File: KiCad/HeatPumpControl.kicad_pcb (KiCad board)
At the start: 2 copper layers, 36.6 x 38.9 mm, 43 parts, among them J1 Conn_01x04_Male, J2 Conn_01x04_Male, J3 Conn_01x04_Male, J4 Conn_01x03_Male, Q1 2N2222A, Q2 Q_PMOS_GDS, U3 XIAO-ESP32-C6-SMD

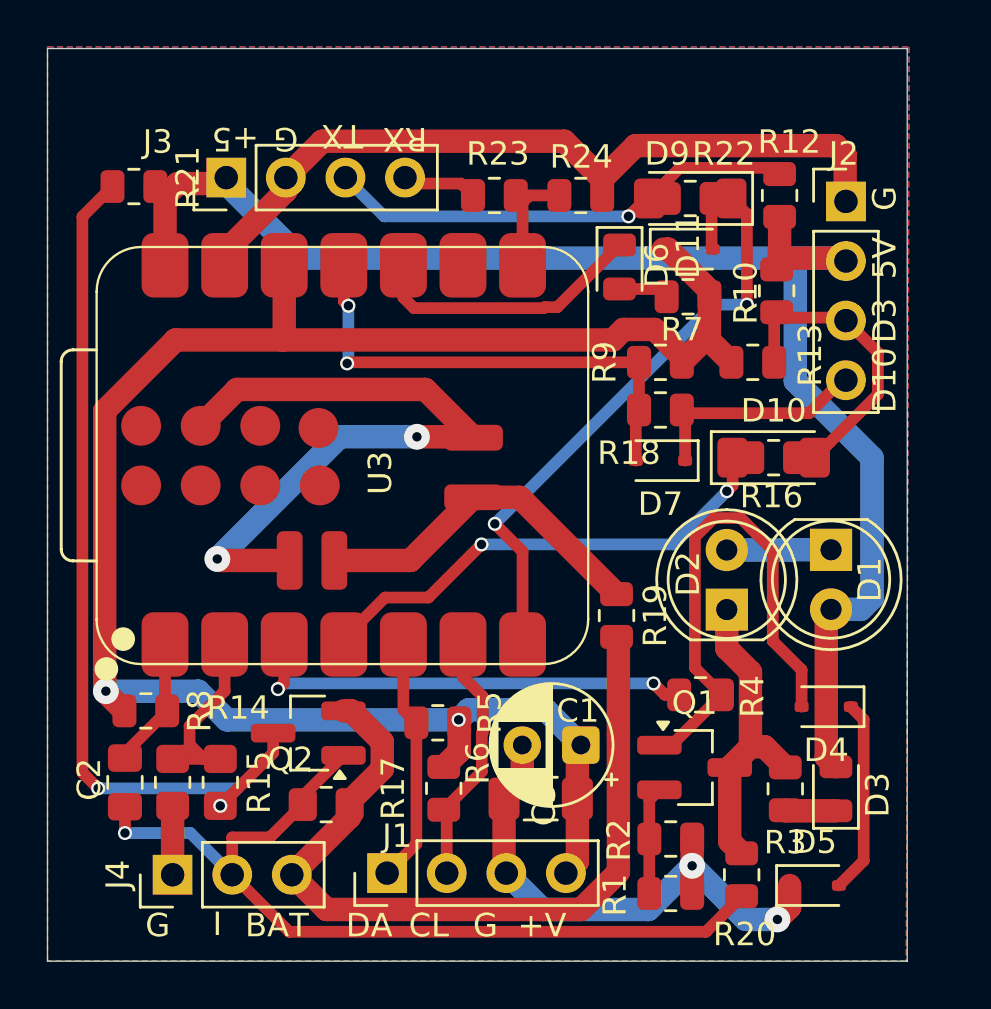
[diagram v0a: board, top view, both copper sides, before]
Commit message: Manufacturing for v4.0
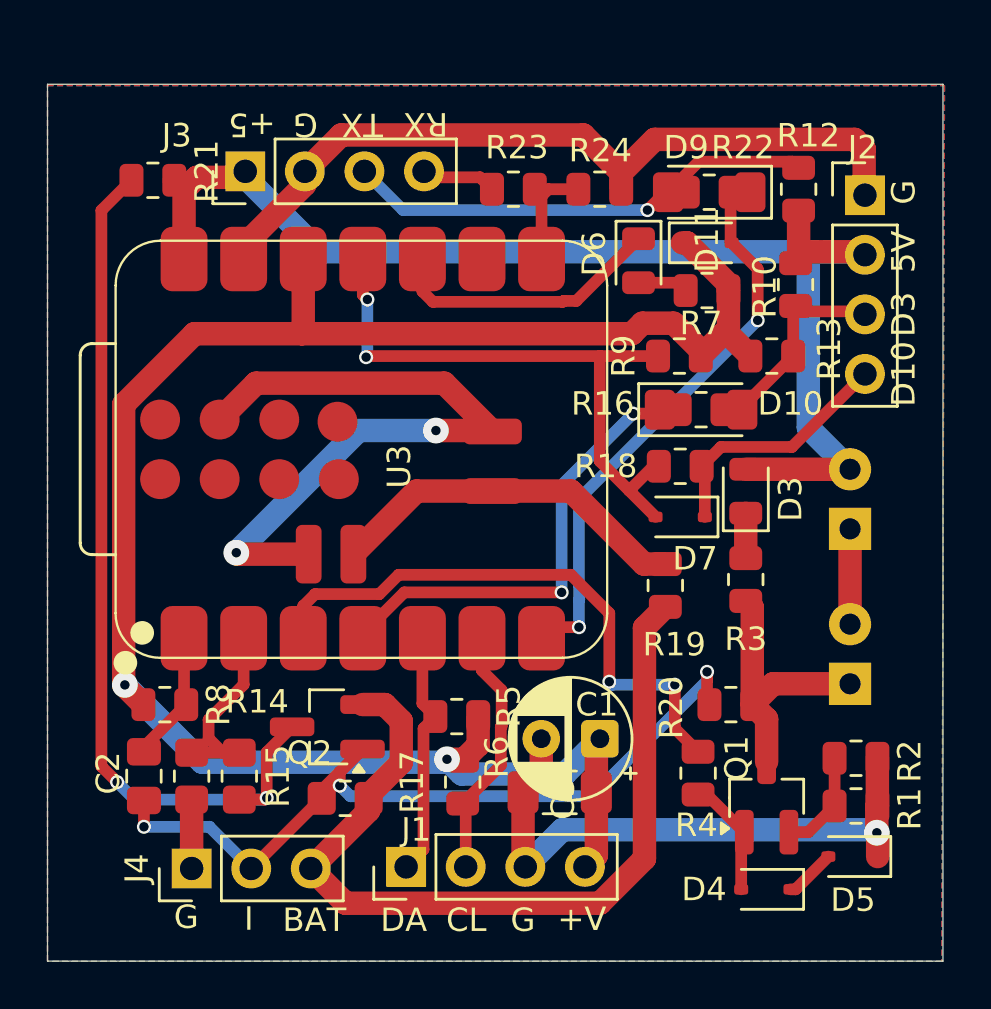
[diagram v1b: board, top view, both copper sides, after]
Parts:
- D1, D2: moved to B.Cu
- moved D3 13.3 mm to (165.7, 103.8)
- moved R3 9.08 mm to (165.7, 107.6), turned to 90 degrees
- moved R1 8.73 mm to (170.4, 117.2)
- moved R2 8.62 mm to (170.4, 115.2)
- moved D4 8.20 mm to (166.5, 120.8)
- moved R20 7.27 mm to (165.0, 112.9), turned to 0 degrees
- moved D2 6.13 mm to (170.1, 112.0)
- moved D10 3.71 mm to (163.8, 100.3)
- moved R16 3.71 mm to (163.8, 100.3)
- moved R4 3.34 mm to (163.6, 115.8), turned to -90 degrees
- moved Q1 3.32 mm to (166.5, 116.8), turned to 90 degrees
- moved D7 2.54 mm to (162.9, 104.9)
- moved R18 2.54 mm to (162.9, 102.7)
- moved R19 2.44 mm to (162.2, 107.8)
- moved D5 2.06 mm to (170.2, 119.4), turned to 180 degrees
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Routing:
- net Net-(D4-A): track 22.2 -> 5.13 mm
- net +5V: track 63.9 -> 53.6 mm
- net Net-(D4-K): track 8.28 -> 2.20 mm
- net /D10: track 21.0 -> 26.3 mm
- net /D2: track 19.4 -> 24.7 mm
- net Net-(D10-A): track 13.6 -> 8.38 mm
- net /TX: track 28.1 -> 24.8 mm
- net Net-(J4-Pin_2): track 37.8 -> 35.2 mm, vias 1 -> 3
- net GND: track 89.3 -> 91.3 mm, vias 4 -> 3
- net +VBAT: track 34.7 -> 36.6 mm
- net +3V3: track 80.3 -> 81.9 mm
- net /ON: track 13.2 -> 11.8 mm
- net /D3: track 21.5 -> 20.3 mm
- net Net-(D7-K): track 9.68 -> 10.8 mm
- net /BAT: track 14.9 -> 15.7 mm
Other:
- board size 36.6 x 38.9 mm -> 38.2 x 37.4 mm
